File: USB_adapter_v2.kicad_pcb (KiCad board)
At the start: 2 copper layers, 46 x 33 mm, 24 parts, among them IC1 AP2112M-3.3TRG1, J1 10033527-N3112MLF, J2 Conn_02x10_Odd_Even, J3 Conn_01x05, J4 Standard?, Q1 BC847BDW1, SW1 PTS526_SK15_SMTR2_LFS, U1 CP2102NP1174GM, U2 D1213A-02SM

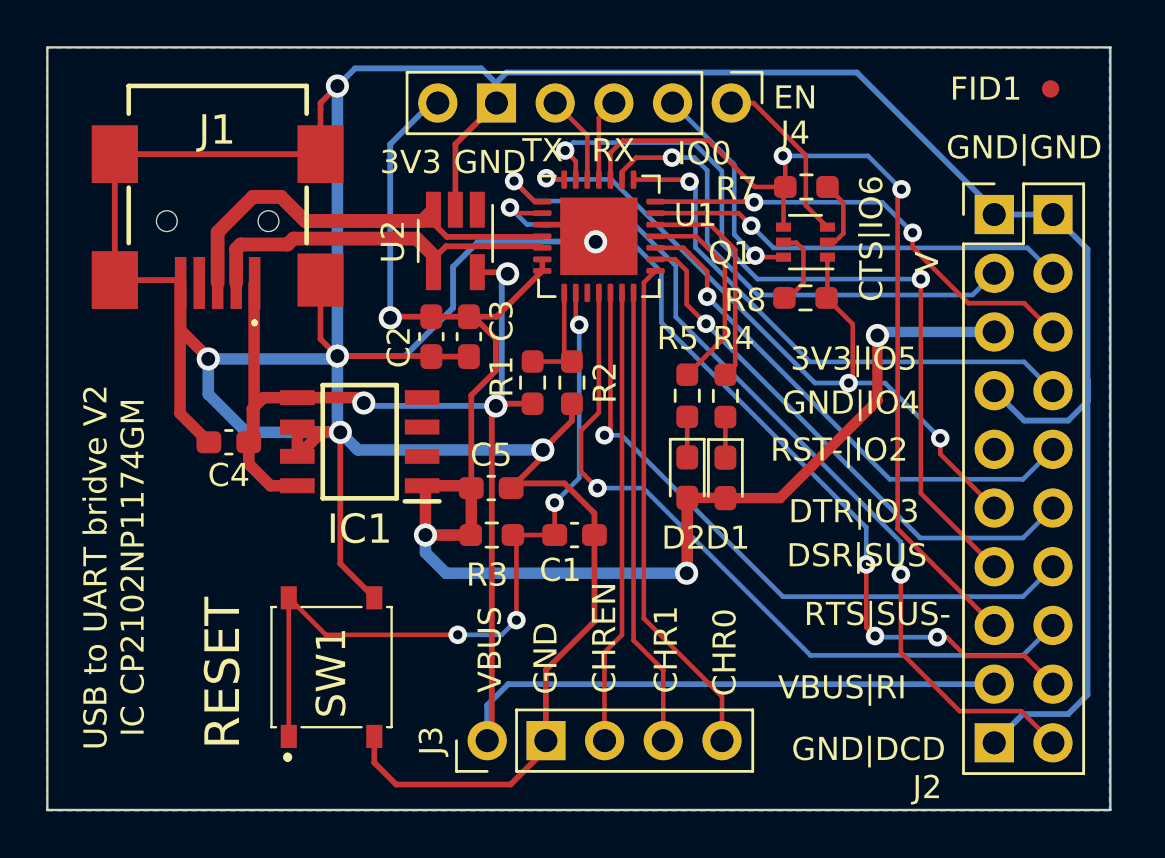
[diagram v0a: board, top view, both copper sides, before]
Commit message: g
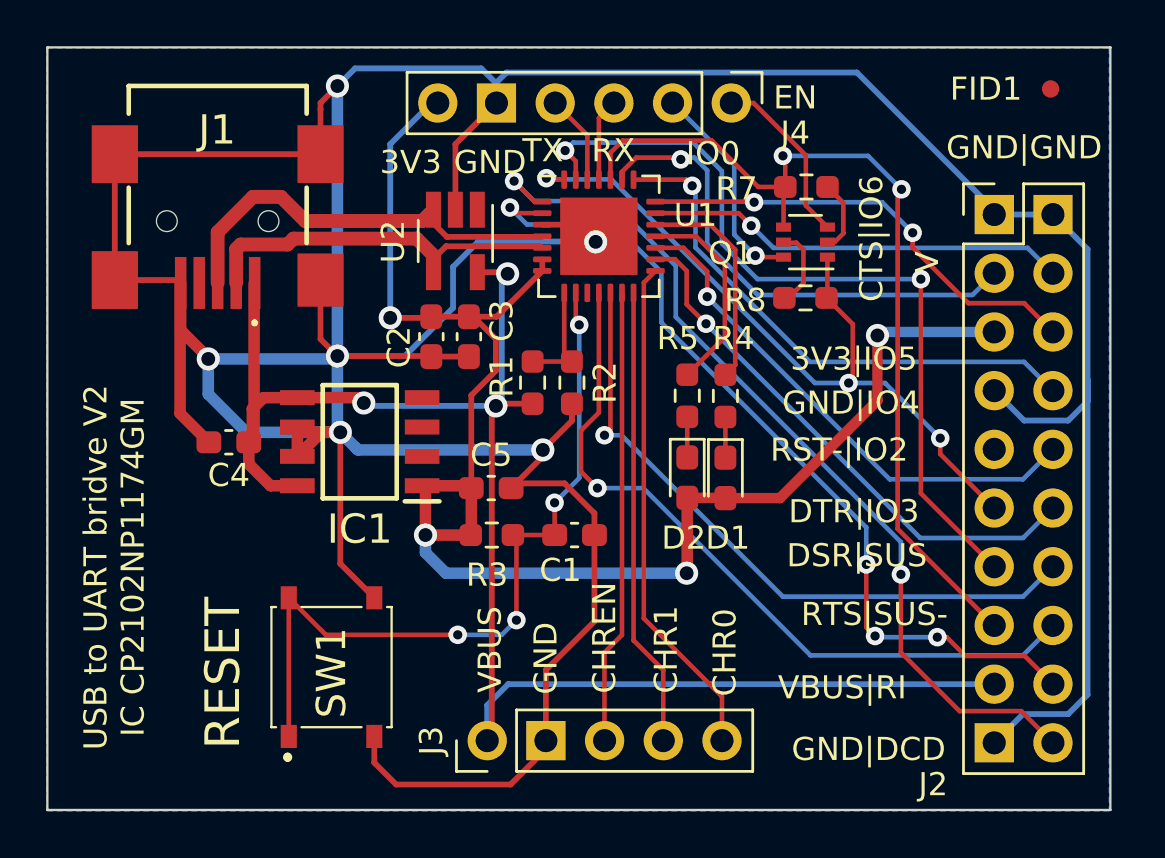
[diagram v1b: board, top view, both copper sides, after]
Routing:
- net GND: track 214.8 -> 212.9 mm
- net VBUS: track 70.5 -> 70.0 mm
- net /EN: track 8.16 -> 7.66 mm

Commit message: f
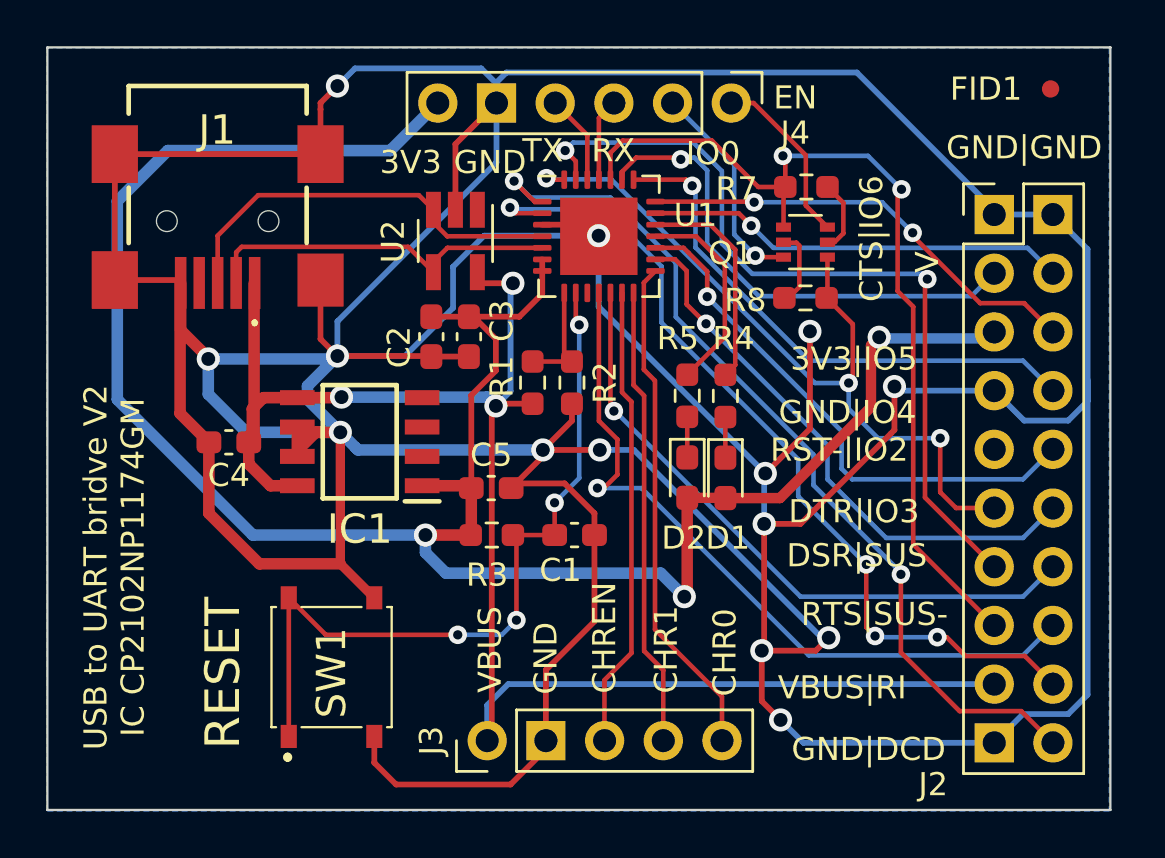
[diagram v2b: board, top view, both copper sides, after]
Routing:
- net GND: track 212.9 -> 298.1 mm, vias 6 -> 14
- net +3V3: track 68.7 -> 96.5 mm, vias 4 -> 3
- net /DTR: track 32.4 -> 34.1 mm
- net /SUSPEND: track 29.1 -> 28.0 mm
- net /GPIO2: track 22.5 -> 23.5 mm
- net D-: track 16.8 -> 15.8 mm
- net /GPIO3: track 23.6 -> 24.4 mm

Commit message: f
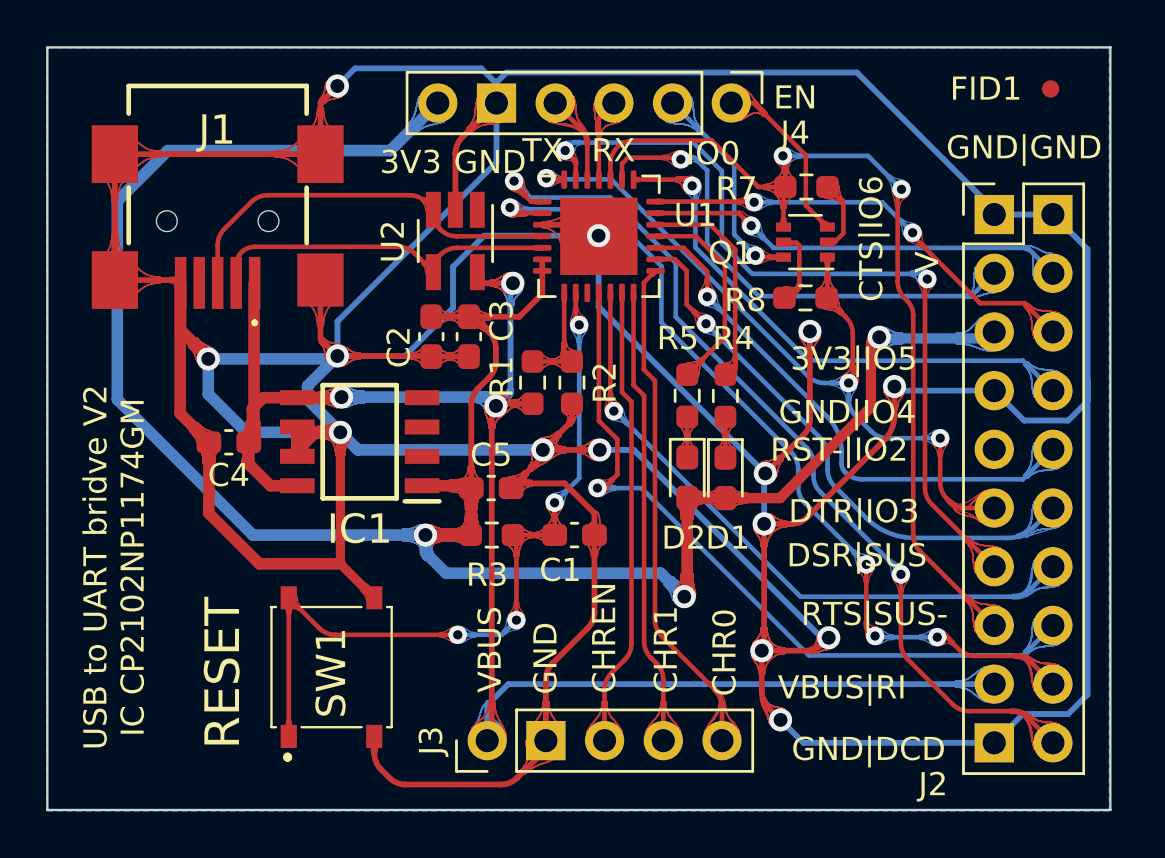
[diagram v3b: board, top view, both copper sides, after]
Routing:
- net GND: track 298.1 -> 297.5 mm
